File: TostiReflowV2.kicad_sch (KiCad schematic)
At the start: 28 parts, among them IC1 CP2102C-A01-GQFN24, J1 USB-C USB2.0 14Pin, Q1 BC817-40, Q2 BC817-40, SW1 EN, SW2 BOOT, U1 ESP32-S3-WROOM-1-N8R2, U5 AMS1117-3.3

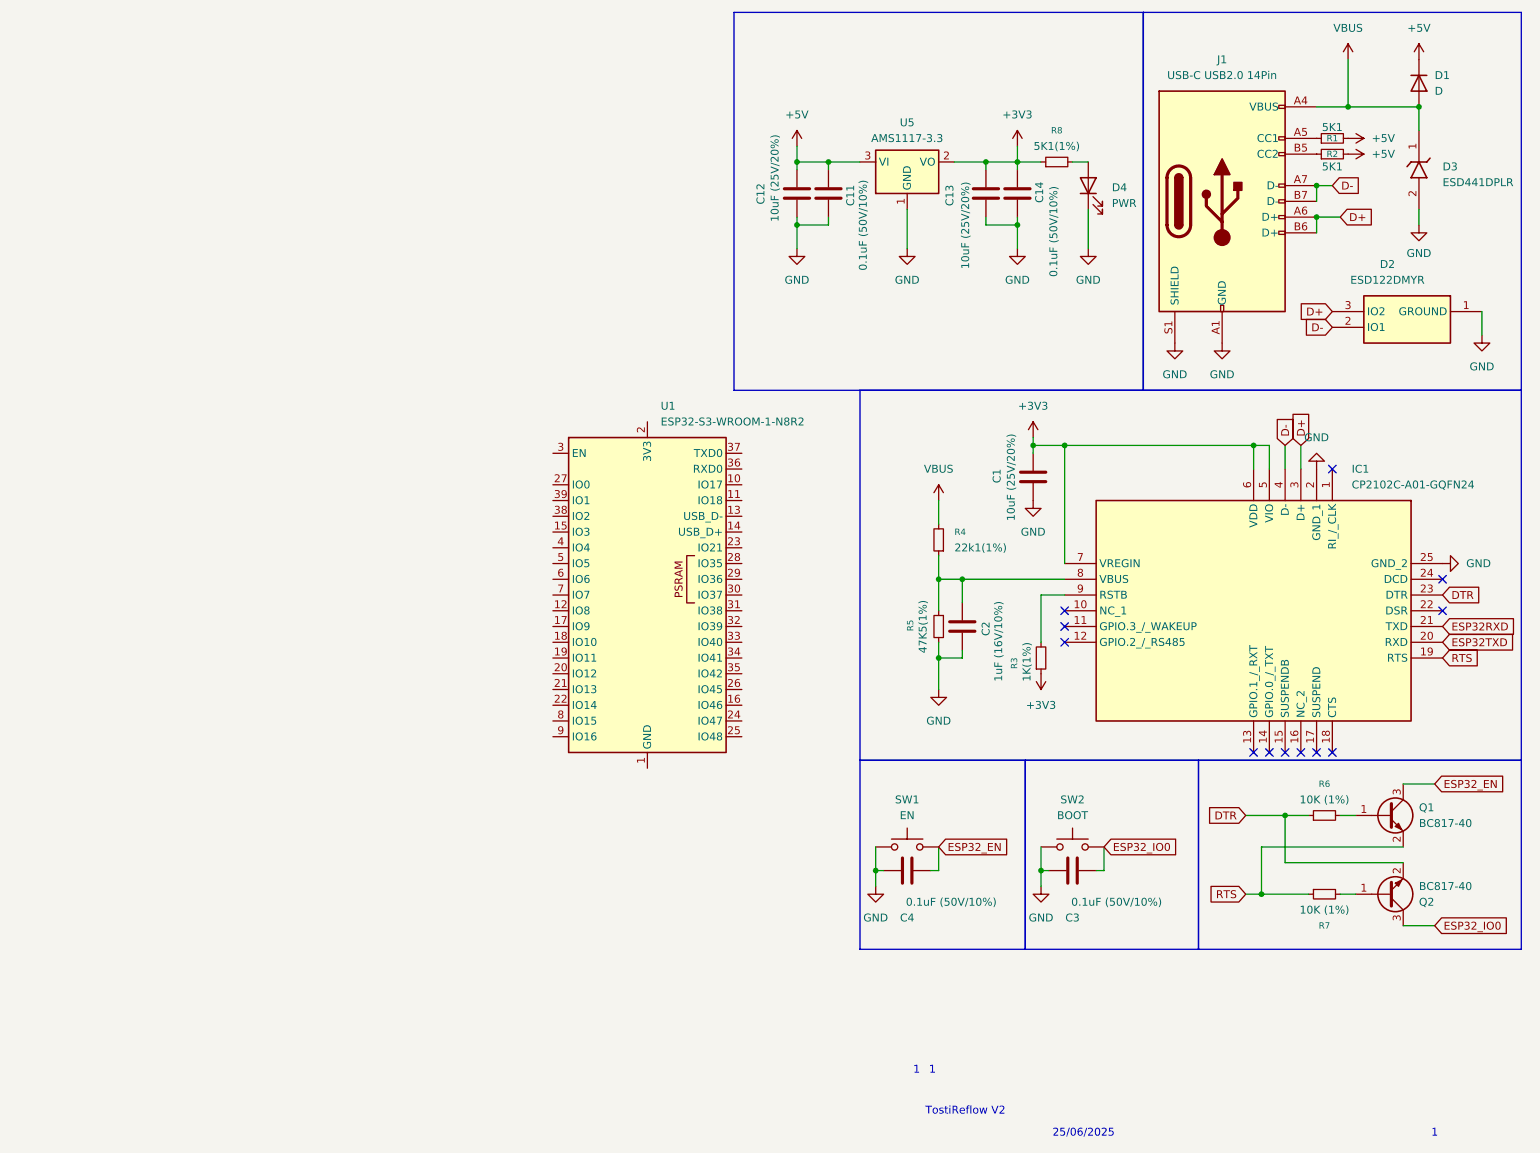
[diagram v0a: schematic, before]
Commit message: Cont.
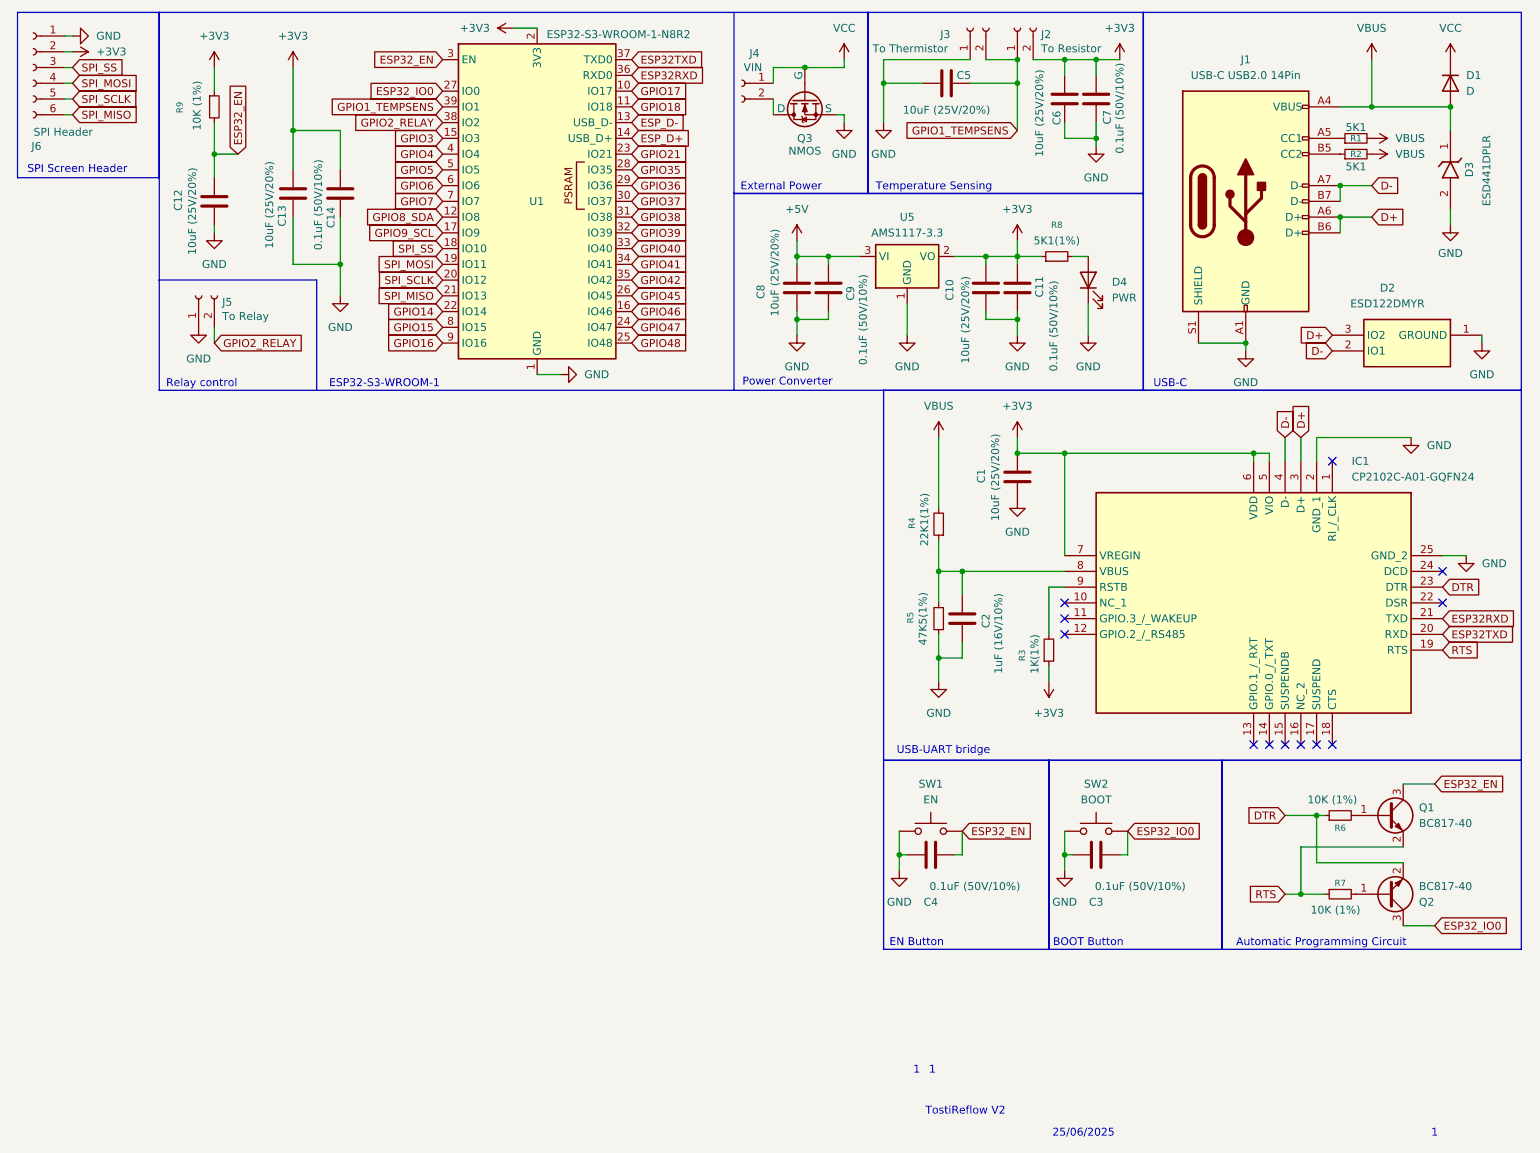
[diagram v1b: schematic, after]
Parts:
- added C12, C13, C5, C6: 10uF (25V/20%), symbol Device:C
- added C14, C7: 0.1uF (50V/10%), Capacitor_SMD:C_0603_1608Metric, symbol Device:C
- added J2: To Resistor, Connector_PinSocket_2.54mm:PinSocket_1x02_P2.54mm_Vertical, symbol Connector:Conn_01x02_Socket
- added J3: To Thermistor, Connector_PinSocket_2.54mm:PinSocket_1x02_P2.54mm_Vertical, symbol Connector:Conn_01x02_Socket
- added J4: VIN, Connector_PinSocket_2.54mm:PinSocket_1x02_P2.54mm_Vertical, symbol Connector:Conn_01x02_Socket
- added J5: To Relay, symbol Connector:Conn_01x02_Socket
- added J6: SPI Header, Connector_PinSocket_2.54mm:PinSocket_1x06_P2.54mm_Vertical, symbol Connector:Conn_01x06_Socket
- added Q3: NMOS, symbol Simulation_SPICE:NMOS
- added R9: 10K (1%), symbol Device:R_Small
- R4: value 22k1(1%) -> 22K1(1%)
- renumbered C13 to C10, C14 to C11, C12 to C8, C11 to C9
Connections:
- net +3V3: now also U1.2 (3V3), C13.1, C14.1, C6.2, C7.2, J2.2 (Pin_2), J6.2 (Pin_2), R9.1
- net +5V: no longer D1.1 (K), R1.2, R2.2
- net ESP32RXD: now also U1.36 (RXD0)
- net ESP32TXD: now also U1.37 (TXD0)
- net ESP32_EN: now also U1.3 (EN), C12.1, R9.2
- net ESP32_IO0: now also U1.27 (IO0)
- net GND: now also U1.1 (GND), U1.40 (GND), U1.41 (GND), C12.2, C13.2, C14.2, C5.1, C6.1, C7.1, J3.1 (Pin_1), J5.1 (Pin_1), J6.1 (Pin_1), Q3.3 (S)
- net VBUS: now also R1.2, R2.2
- net GPIO17: now reaches U1.10 (IO17)
- net GPIO18: now reaches U1.11 (IO18)
- net GPIO8_SDA: now reaches U1.12 (IO8)
- net ESP_D-: now reaches U1.13 (USB_D-)
- net ESP_D+: now reaches U1.14 (USB_D+)
- net GPIO3: now reaches U1.15 (IO3)
- net GPIO46: now reaches U1.16 (IO46)
- net GPIO9_SCL: now reaches U1.17 (IO9)
- net SPI_SS: now reaches U1.18 (IO10)
- net SPI_SS: now also J6.3 (Pin_3)
- net SPI_MOSI: now reaches U1.19 (IO11)
- net SPI_MOSI: now also J6.4 (Pin_4)
- net SPI_SCLK: now reaches U1.20 (IO12)
- net SPI_SCLK: now also J6.5 (Pin_5)
- net SPI_MISO: now reaches U1.21 (IO13)
- net SPI_MISO: now also J6.6 (Pin_6)
- net GPIO14: now reaches U1.22 (IO14)
- net GPIO21: now reaches U1.23 (IO21)
- net GPIO47: now reaches U1.24 (IO47)
- net GPIO48: now reaches U1.25 (IO48)
- net GPIO45: now reaches U1.26 (IO45)
- net GPIO35: now reaches U1.28 (IO35)
- net GPIO36: now reaches U1.29 (IO36)
- net GPIO37: now reaches U1.30 (IO37)
- net GPIO38: now reaches U1.31 (IO38)
- net GPIO39: now reaches U1.32 (IO39)
- net GPIO40: now reaches U1.33 (IO40)
- net GPIO41: now reaches U1.34 (IO41)
- net GPIO42: now reaches U1.35 (IO42)
- net GPIO2_RELAY: now reaches U1.38 (IO2)
- net GPIO2_RELAY: now also J5.2 (Pin_2)
- net GPIO1_TEMPSENS: now reaches U1.39 (IO1)
- net GPIO1_TEMPSENS: now also C5.2, J2.1 (Pin_1), J3.2 (Pin_2)
- net GPIO4: now reaches U1.4 (IO4)
- net GPIO5: now reaches U1.5 (IO5)
- net GPIO6: now reaches U1.6 (IO6)
- net GPIO7: now reaches U1.7 (IO7)
- net GPIO15: now reaches U1.8 (IO15)
- net GPIO16: now reaches U1.9 (IO16)
- new net: J4.2 (Pin_2), Q3.1 (D)
- new net VCC: D1.1 (K), J4.1 (Pin_1), Q3.2 (G)
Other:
- note added: "Automatic Programming Circuit"
- note added: "BOOT Button"
- note added: "EN Button"
- note added: "ESP32-S3-WROOM-1"
- note added: "External Power"
- note added: "Power Converter"
- note added: "Relay control"
- note added: "SPI Screen Header"
- note added: "Temperature Sensing"
- note added: "USB-C"
- note added: "USB-UART bridge"
- moved on the sheet: C1, C10, C11, C2, C3, C4, C8, C9, D1, D2, D3, D4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
